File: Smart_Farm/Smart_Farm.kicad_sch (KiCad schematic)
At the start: 30 parts, among them J1 EJ508A, J2 Screw_Terminal_01x03, Q1 2N3904

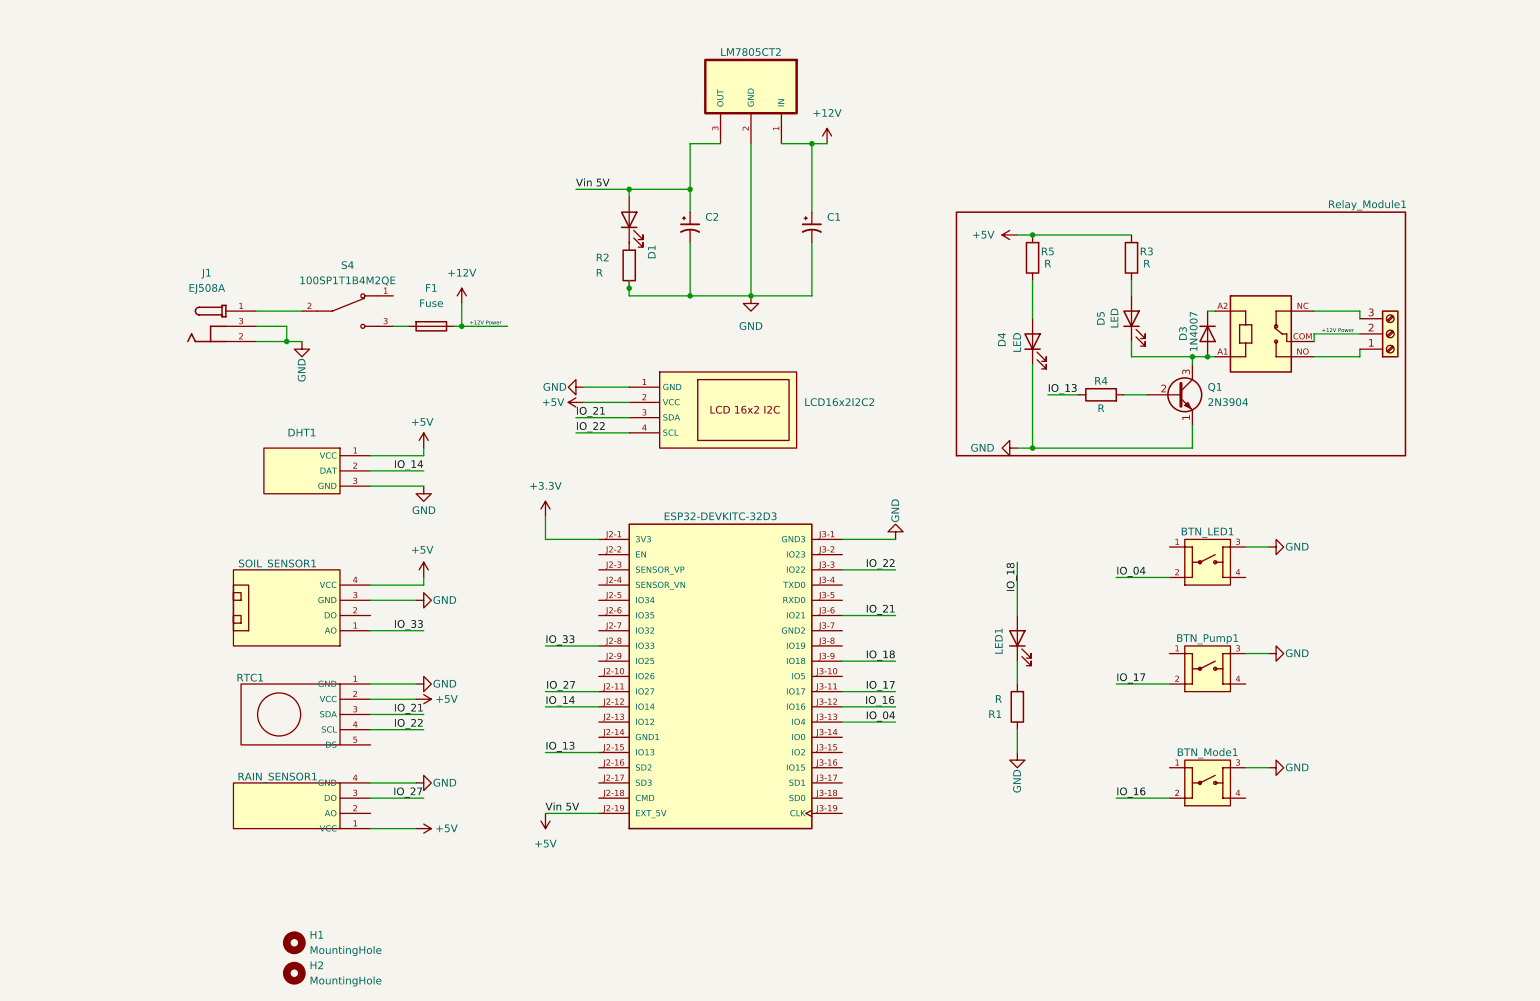
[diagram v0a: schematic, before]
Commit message: Update files
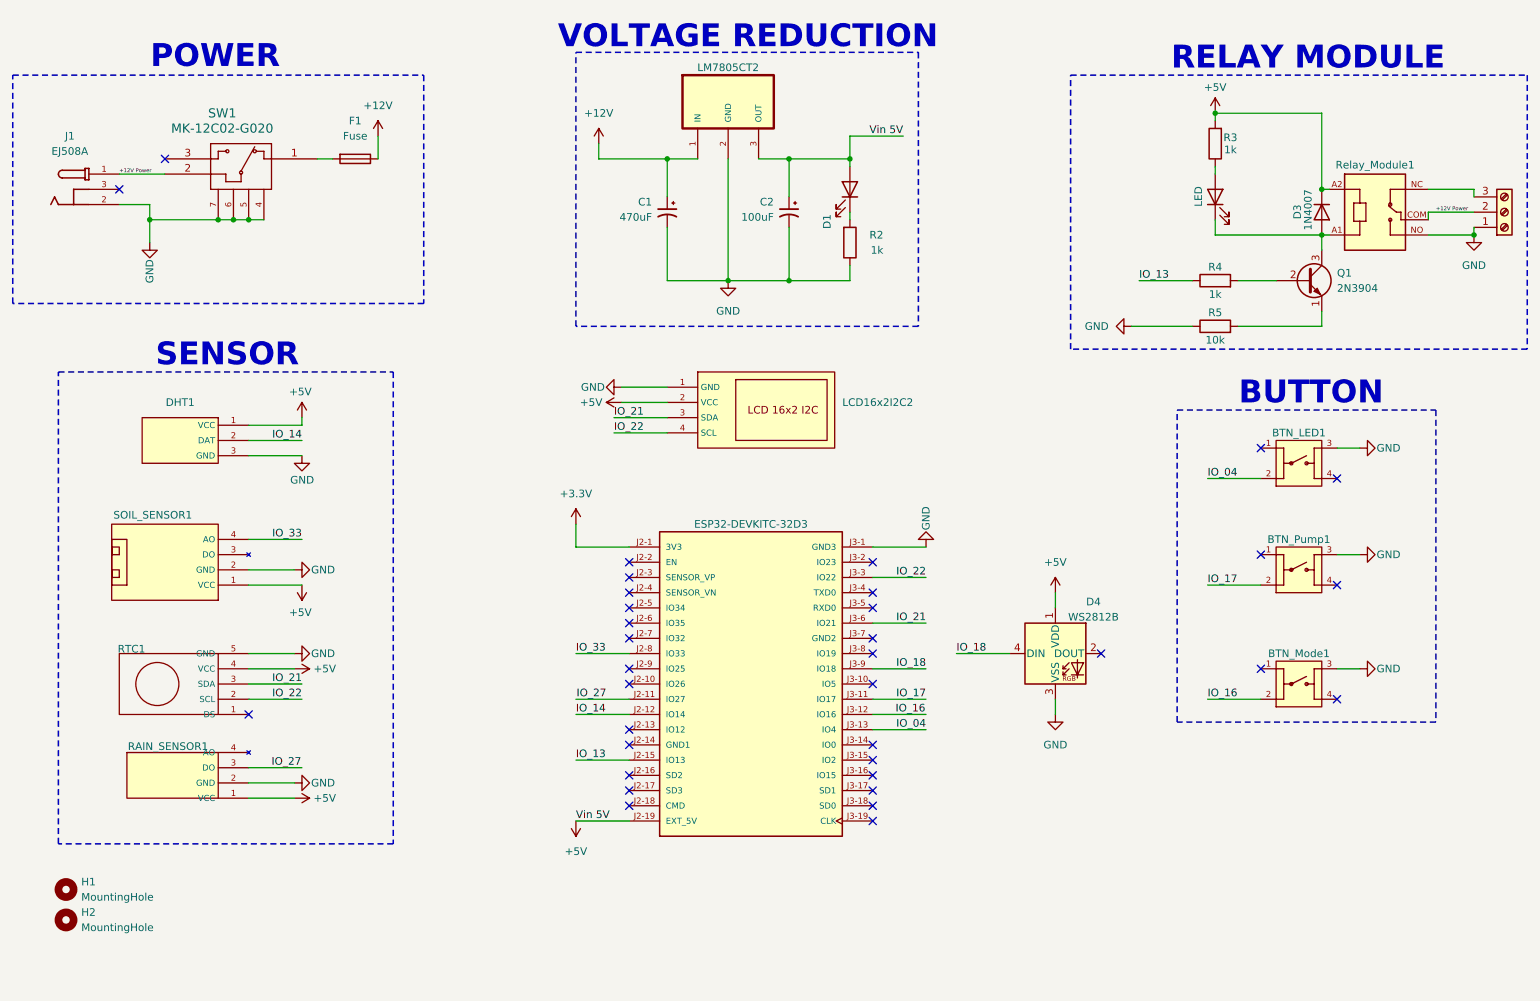
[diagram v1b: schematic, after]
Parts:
- removed D4, LED1: LED, LED_SMD:LED_0805_2012Metric, symbol Device:LED
- removed R1: R, Resistor_SMD:R_0805_2012Metric, symbol Device:R
- removed S4: 100SP1T1B4M2QE, Smart_Farm:SW_100SP1T1B4M2QE, symbol Smart_Farm:100SP1T1B4M2QE
- added D4: WS2812B, LED_SMD:LED_WS2812B_PLCC4_5.0x5.0mm_P3.2mm, symbol LED:WS2812B
- added SW1: MK-12C02-G020, Smart_Farm:MK-12C02-G020_GSW, symbol Smart_Farm:MK-12C02-G020
- C1: value C_Polarized_Small_US -> 470uF
- C2: value C_Polarized_Small_US -> 100uF
- R2, R3, R4: value R -> 1k
- R5: value R -> 10k
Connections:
- net +12V: no longer J2.2 (Pin_2), Relay_Module1.COM
- net +5V: now also D3.1 (K), RTC1.4 (VCC), Relay_Module1.A2, SOIL_SENSOR1.1 (VCC), D4.1 (VDD); no longer R5.2, RTC1.2 (VCC), SOIL_SENSOR1.4 (VCC)
- net GND: now also J2.1 (Pin_1), R5.1, RAIN_SENSOR1.2 (GND), RTC1.5 (GND), Relay_Module1.NO, SOIL_SENSOR1.2 (GND), D4.3 (VSS), SW1.4, SW1.5, SW1.6, SW1.7; no longer J1.3, Q1.1 (E), RAIN_SENSOR1.4 (GND), RTC1.1 (GND), SOIL_SENSOR1.3 (GND)
- net IO_18: now also D4.4 (DIN)
- net IO_22: now also RTC1.2 (SCL); no longer RTC1.4 (SCL)
- net IO_33: now also SOIL_SENSOR1.4 (AO); no longer SOIL_SENSOR1.1 (AO)
- net at F1.2: now also SW1.1
- net +12V Power: now reaches J1.1
- net +12V Power: now also J2.2 (Pin_2), Relay_Module1.COM, SW1.2
- new net: Q1.1 (E), R5.2
- no-connect marks 0 -> 35
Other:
- note added: "BUTTON"
- note added: "POWER"
- note added: "RELAY MODULE"
- note added: "SENSOR"
- note added: "VOLTAGE REDUCTION"
- moved on the sheet: BTN_LED1, BTN_Mode1, BTN_Pump1, C1, C2, D1, D3, DHT1, ESP32-DEVKITC-32D3, F1, H1, H2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
